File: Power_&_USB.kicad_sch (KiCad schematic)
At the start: 37 parts, among them J5 USB4745-03-A, U10 93LC66B-I/MS, U11 93LCxxA, U12 SN74LVC1T45DCK, U4 FT232HPQ, U6 SN74AXC4T774RSVR, Y2 ASCO-12.000MHZ-EK-T3

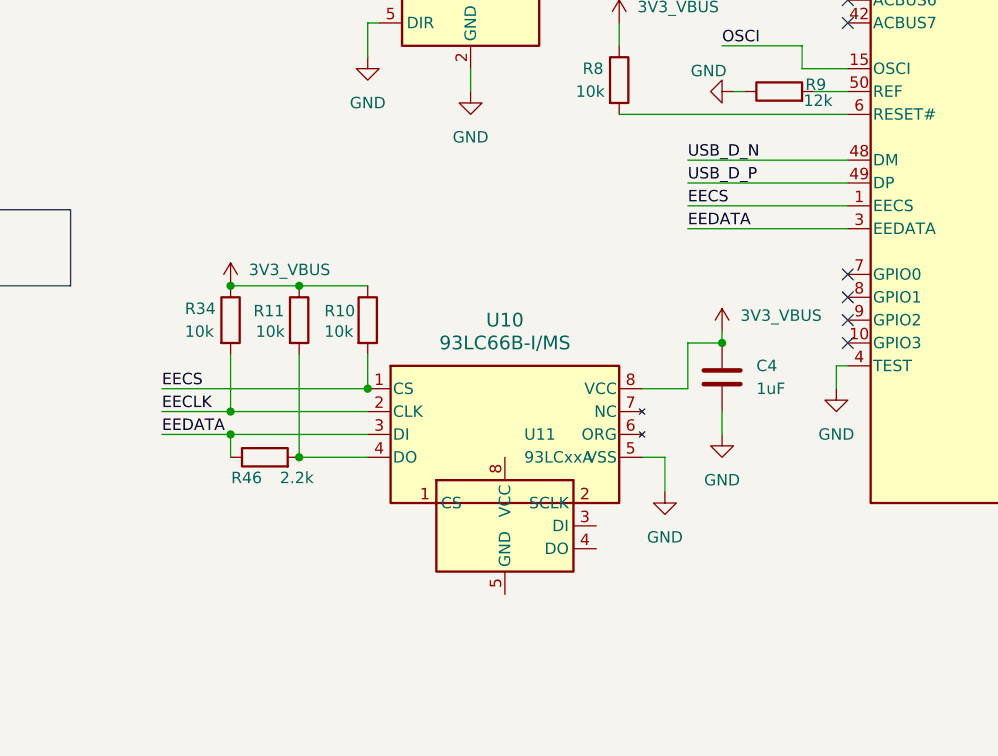
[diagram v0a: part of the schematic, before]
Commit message: updated routing
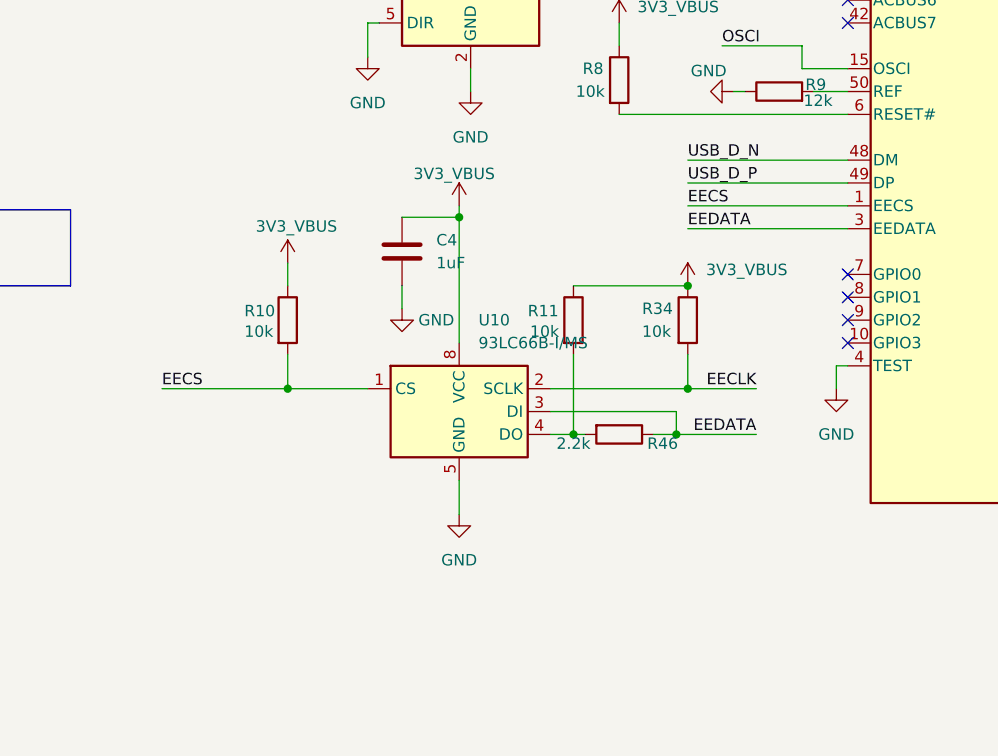
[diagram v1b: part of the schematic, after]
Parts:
- removed U11: 93LCxxA, Package_SO:SOIC-8_3.9x4.9mm_P1.27mm, symbol Memory_EEPROM:93LCxxA
- Y2: footprint dz_comm:ASCO16000MHZEKT -> Oscillator:Oscillator_SMD_Abracon_ASCO-4Pin_1.6x1.2mm
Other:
- moved on the sheet: C4, R10, R11, R34, R46
